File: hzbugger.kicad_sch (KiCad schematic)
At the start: 50 parts, among them J2 IDC, J4 SWD, J6 GPIO, SW1 RESET_SW, U1 STM32F103C8T6, U2 SRV05-4, U3 AMS1117-3.3, U4 HX AM 90D, Y1 8M

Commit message: w.i.p
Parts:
- J2: footprint Connector_IDC:IDC-Header_2x05_P2.54mm_Vertical -> hzbugger:SMD-pcbend-IDC-Header_2x05_P2.54mm
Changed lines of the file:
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@@
 			)
 		)
-		(property "Footprint" "Connector_IDC:IDC-Header_2x05_P2.54mm_Vertical"
+		(property "Footprint" "hzbugger:SMD-pcbend-IDC-Header_2x05_P2.54mm"
 			(at 196.85 134.62 0)
 			(effects

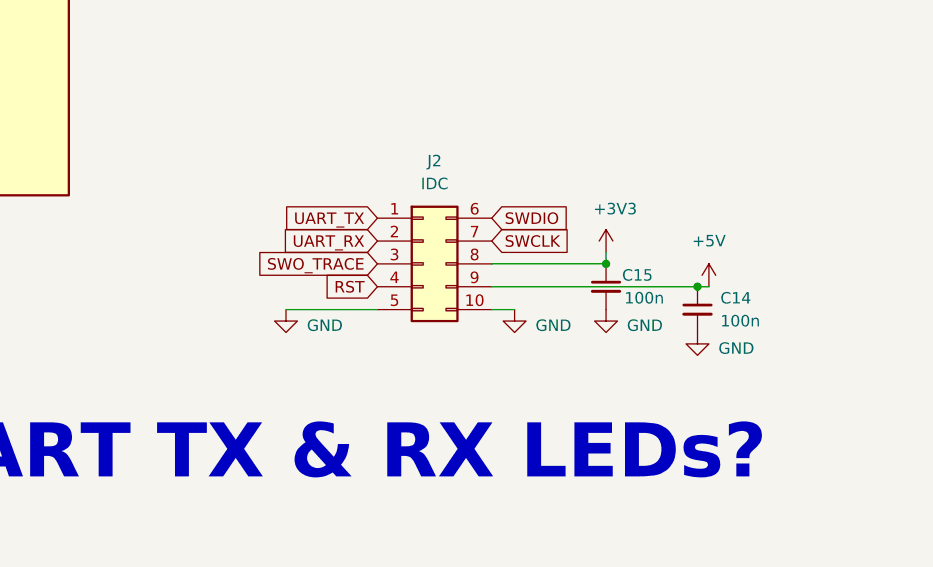
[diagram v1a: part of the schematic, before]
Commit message: IDC
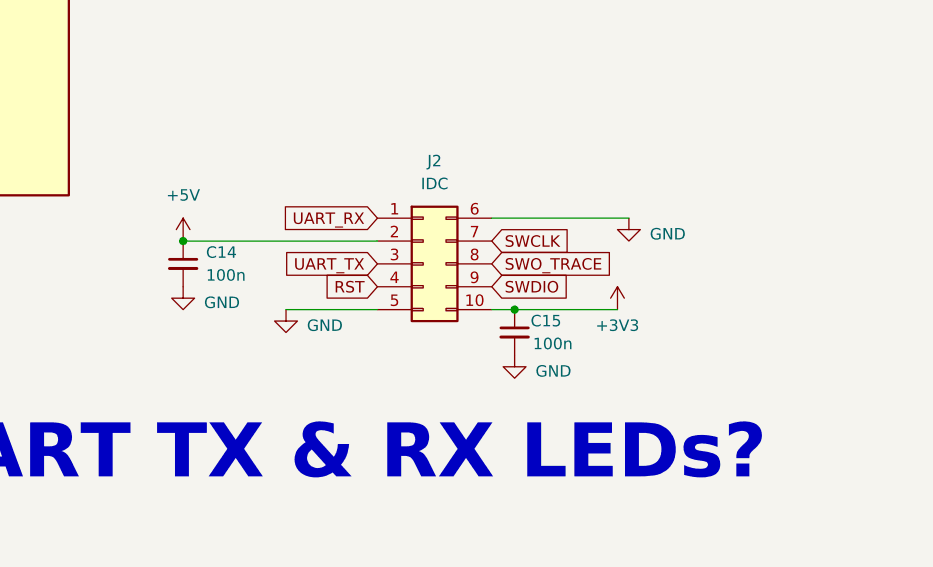
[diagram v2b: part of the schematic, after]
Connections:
- net +3V3: now also J2.10 (Pin_10); no longer J2.8 (Pin_8)
- net +5V: now also J2.2 (Pin_2); no longer J2.9 (Pin_9)
- net GND: now also J2.6 (Pin_6); no longer J2.10 (Pin_10)
- net SWDIO: now also J2.9 (Pin_9); no longer J2.6 (Pin_6)
- net SWO_TRACE: now also J2.8 (Pin_8); no longer J2.3 (Pin_3)
- net UART_RX: now also J2.1 (Pin_1); no longer J2.2 (Pin_2)
- net UART_TX: now also J2.3 (Pin_3); no longer J2.1 (Pin_1)
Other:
- moved on the sheet: C14, C15
